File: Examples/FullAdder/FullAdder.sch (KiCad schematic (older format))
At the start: 13 parts, among them U1 plot_v1, U2 plot_v1, U3 plot_v1, U4 plot_v1, U5 plot_v1, U6 adc_bridge_3, U7 dac_bridge_2, X1 full_adder

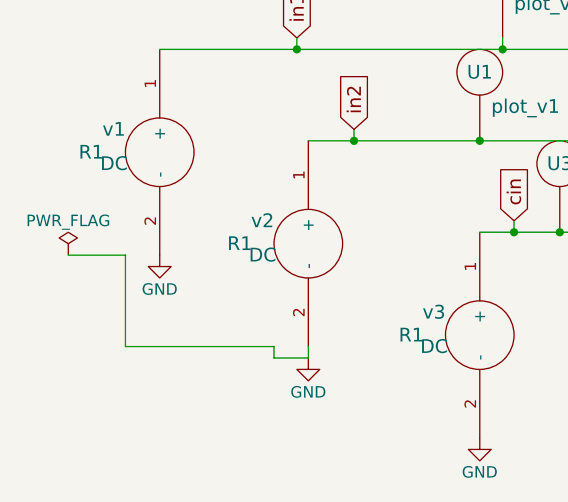
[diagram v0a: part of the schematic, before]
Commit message: Examples pulled from original
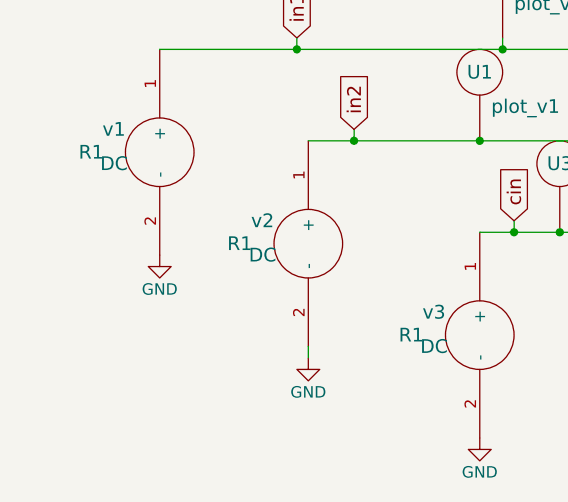
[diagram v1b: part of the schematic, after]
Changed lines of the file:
@@
 LIBS:74xx
 LIBS:cmos4000
-LIBS:FullAdder-cache
 EELAYER 25 0
 EELAYER END
@@
 Wire Wire Line
 	1950 4400 1950 4450
-$Comp
-L PWR_FLAG #FLG06
-U 1 1 5CEE2E64
-P 900 4000
-F 0 "#FLG06" H 900 4075 50  0001 C CNN
-F 1 "PWR_FLAG" H 900 4150 50  0000 C CNN
-F 2 "" H 900 4000 50  0001 C CNN
-F 3 "" H 900 4000 50  0001 C CNN
-	1    900  4000
-	1    0    0    -1
-$EndComp
-Wire Wire Line
-	900  4000 1150 4000
-Wire Wire Line
-	1150 4000 1150 4400
-Wire Wire Line
-	1150 4400 1800 4400
-Wire Wire Line
-	1800 4400 1800 4450
-Wire Wire Line
-	1800 4450 1950 4450
 $EndSCHEMATC
